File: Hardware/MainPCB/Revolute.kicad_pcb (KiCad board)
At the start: 4 copper layers, 16.8 x 11.4 mm, 32 parts, among them J1 USB_A, U1 nRF52840_aQFN73, U3 AP2112K-3.3, U4 debug_ports, X1 32MHZ, X2 32.768 kHz

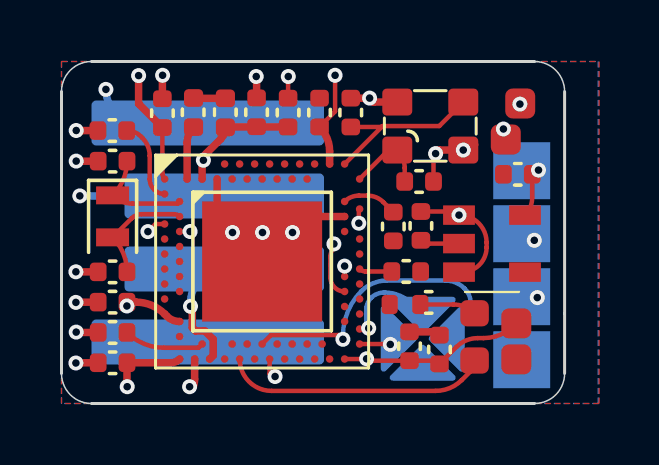
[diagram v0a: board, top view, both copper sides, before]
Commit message: made pcb smaller
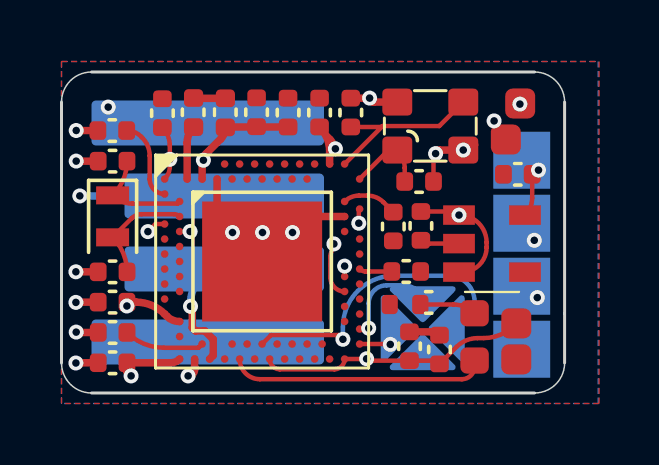
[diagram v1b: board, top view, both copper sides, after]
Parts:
- moved U4 0.35 mm to (172.5, 81.6)
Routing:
- net VBUS: track 32.9 -> 30.0 mm
- net GND: track 19.9 -> 17.6 mm, vias 15 -> 12
- net VDD_nRF: track 18.0 -> 17.1 mm, vias 6 -> 5
- net Net-(J1-D-): track 13.6 -> 12.8 mm
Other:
- board size 16.8 x 11.4 mm -> 16.8 x 10.7 mm
